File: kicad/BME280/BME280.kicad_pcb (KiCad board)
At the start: 2 copper layers, 5 x 6.9 mm, 8 parts, among them J1 Conn, J2 Conn, J3 Conn, J4 Conn, U1 BME280

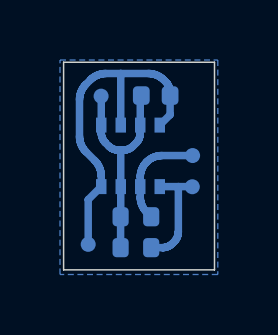
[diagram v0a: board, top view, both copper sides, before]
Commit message: новый файл:    Documents/IMG_20230122_160000.png 	изменено:      kicad/BME280/BME280.kicad_pcb 	изменено:      kicad/BME280/BME280.kicad_pcb-bak
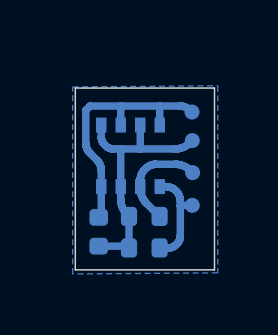
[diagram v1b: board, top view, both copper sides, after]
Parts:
- moved J4 5.61 mm to (37.2, 40.4)
- moved C1 4.92 mm to (34.1, 44.4), turned to 90 degrees
- moved J1 3.38 mm to (37.2, 41.4)
- moved J2 0.62 mm to (37.2, 43.5)
- moved J3 0.57 mm to (37.2, 42.4)
- moved R1 0.28 mm to (35.6, 44.9)
- moved R2 0.28 mm to (35.6, 43.9)
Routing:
- net Gnd: track 12.0 -> 8.71 mm
- net Vcc: track 7.67 -> 8.96 mm
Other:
- board size 5 x 6.9 mm -> 4.6 x 6.1 mm

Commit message: изменено:      FreeCAD/GM_case.FCStd 	изменено:      kicad/BME280/BME280.kicad_pcb 	изменено:      kicad/Meteostation_4/Meteostation-rescue.lib 	изменено:      kicad/Meteostation_4/Meteostation.kicad_pcb 	изменено:      stm32cubeide/Meteostation/.settings/language.settings.xml 	изменено:      stm32cubeide/Meteostation/Core/Inc/main.h 	изменено:      stm32cubeide/Meteostation/Core/Src/main.c 	изменено:      stm32cubeide/Meteostation/Meteostation.ioc 	изменено:      stm32cubeide/Meteostation/Meteostation.launch 	изменено:      stm32cubeide/Meteostation/Release/Core/Src/main.o 	изменено:      stm32cubeide/Meteostation/Release/Core/Src/main.su 	изменено:      stm32cubeide/Meteostation/Release/Core/Src/stm32f1xx_it.o 	изменено:      stm32cubeide/Meteostation/Release/Meteostation.bin 	изменено:      stm32cubeide/Meteostation/Release/Meteostation.elf 	изменено:      stm32cubeide/Meteostation/Release/Meteostation.hex 	изменено:      stm32cubeide/Meteostation/Release/Meteostation.list 	изменено:      stm32cubeide/Meteostation/Release/Meteostation.map
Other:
- net class Default removed
